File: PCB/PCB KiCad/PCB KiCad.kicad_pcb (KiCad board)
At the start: 2 copper layers, 40 x 40 mm, 57 parts, among them J1 Conn_01x04, J2 Qwiic, J3 Conn_01x04, J4 Conn_01x04, J5 Conn_01x04, U1 OPA2376AID, U2 NAU7802SGI, U3 TLC59208FIPWR

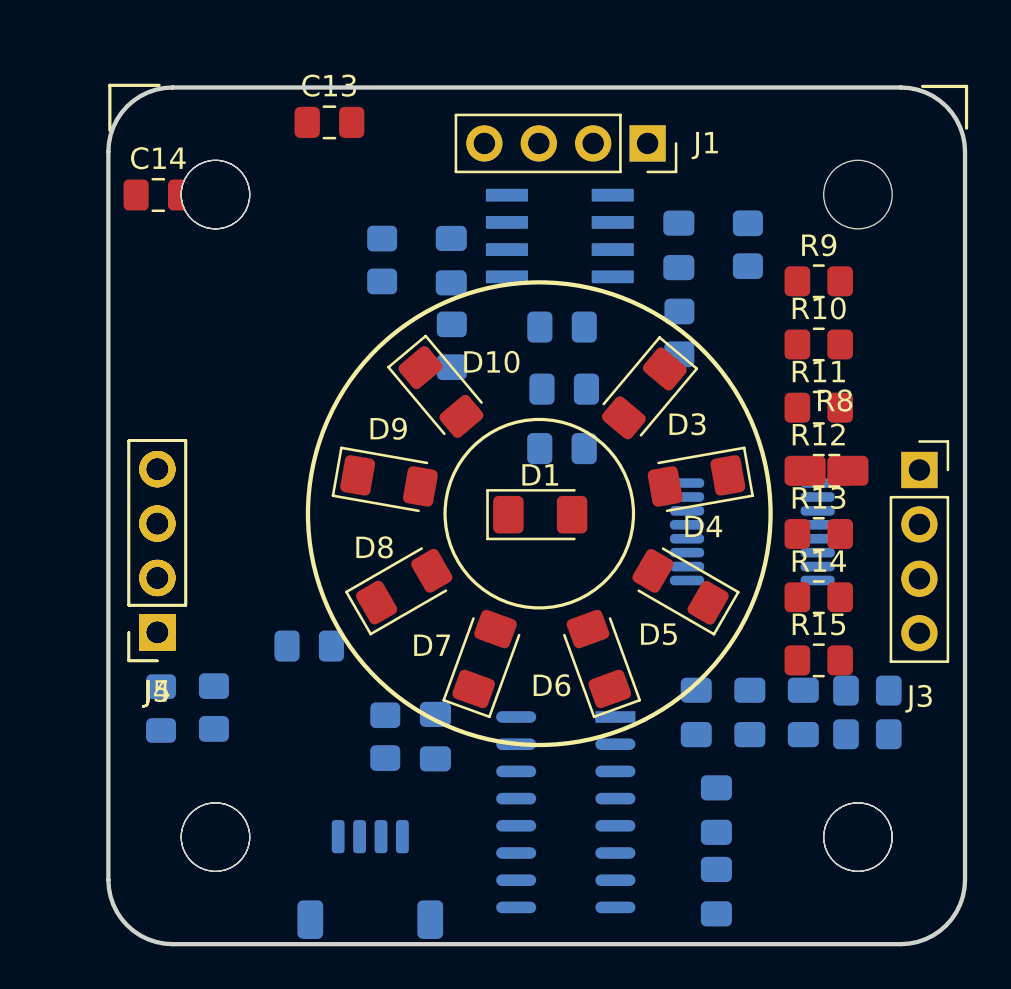
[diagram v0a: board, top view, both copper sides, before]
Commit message: routed!
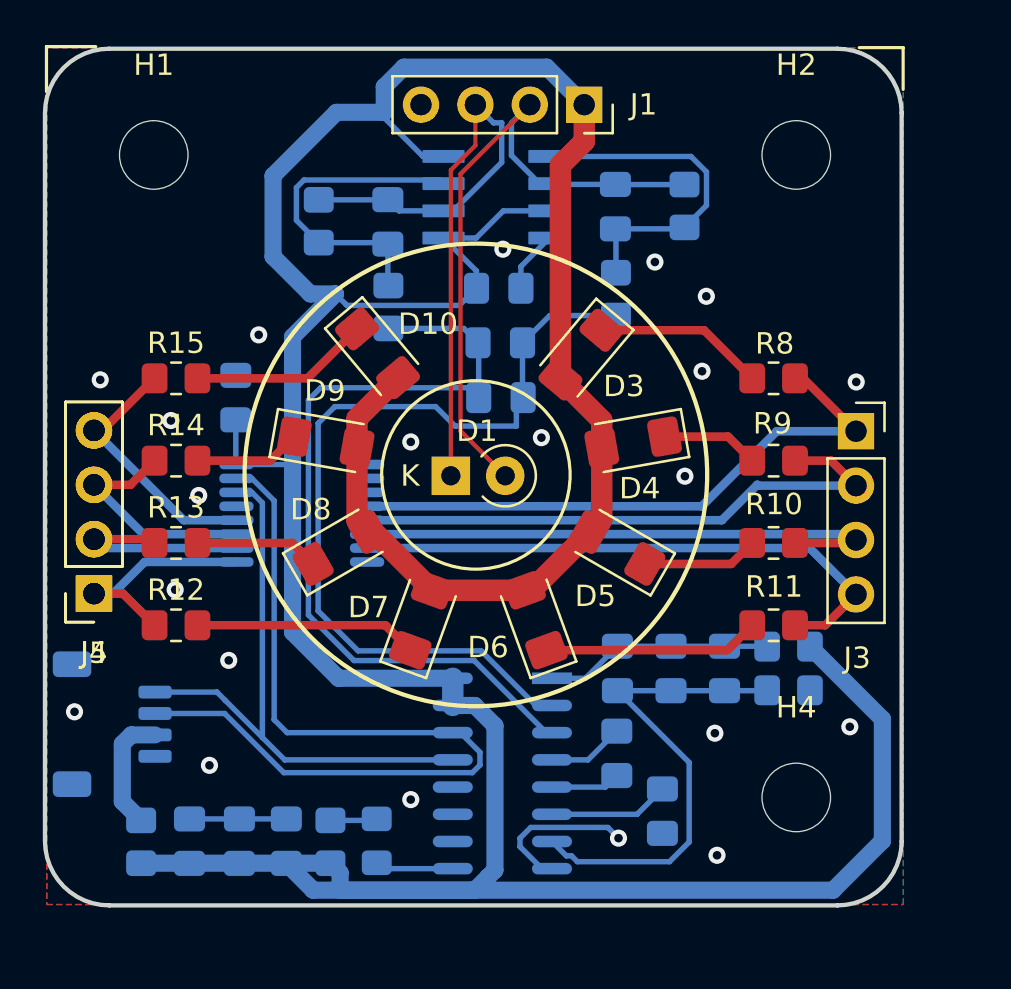
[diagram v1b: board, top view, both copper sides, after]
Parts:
- removed ? (x3): , 
- removed H3: MountingHole, MountingHole:MountingHole_3.2mm_M3
- C13, C14: moved to B.Cu
- D1: footprint Diode_SMD:D_1206_3216Metric_Pad1.42x1.75mm_HandSolder -> Diode_THT:D_A-405_P2.54mm_Vertical_KathodeUp
- moved H2 41.8 mm to (95.0, 120.0)
- moved C13 33.8 mm to (69.0, 152.0), turned to 90 degrees
- moved R15 32.8 mm to (66.0, 130.4)
- moved R12 30.9 mm to (66.0, 142.0)
- moved R14 30.7 mm to (66.0, 134.3)
- moved R13 30.0 mm to (66.0, 138.1)
- moved H4 28.3 mm to (95.0, 150.0)
- moved U3 21.1 mm to (71.9, 136.7)
- moved J2 14.1 mm to (63.1, 146.6), turned to 90 degrees
- moved C10 12.5 mm to (66.7, 152.0), turned to 90 degrees
- moved FB1 12.4 mm to (64.4, 152.1), turned to 90 degrees
- moved D2 11.8 mm to (75.4, 152.0), turned to 90 degrees
- moved R11 10.4 mm to (93.9, 142.0), turned to 180 degrees
- moved C14 10.1 mm to (68.8, 131.3), turned to 90 degrees
- moved R10 9.50 mm to (93.9, 138.1), turned to 180 degrees
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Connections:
- R7 pad 1: 3v3unf -> 3.3v
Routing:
- net 3.3v: track 0.00 -> 184.9 mm
- net /ADC/AIN-: track 0.00 -> 40.4 mm
- net SDA: track 0.00 -> 39.7 mm
- net /ADC/AIN+: track 0.00 -> 39.1 mm
- net /Sensor/A-: track 0.00 -> 30.9 mm
- net /Sensor/A+: track 0.00 -> 30.9 mm
- net LED1: track 0.00 -> 28.2 mm
- net SCL: track 0.00 -> 27.6 mm
- net LED4: track 0.00 -> 27.2 mm
- net LED2: track 0.00 -> 26.9 mm
- net LED3: track 0.00 -> 25.9 mm
- net Net-(U2-REFN): track 0.00 -> 22.7 mm
- net GND: track 0.00 -> 18.4 mm, vias 0 -> 21
- net Net-(U1-OUT_A): track 0.00 -> 16.0 mm
- net Net-(U1-OUT_B): track 0.00 -> 15.3 mm
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- added copper zone on B.Cu, net GND
- added copper zone on F.Cu, net GND
